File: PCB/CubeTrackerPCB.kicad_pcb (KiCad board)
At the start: 2 copper layers, 28 x 50.9 mm, 9 parts, among them U1 XIAO-RP2040-DIP, U2 ICM-42688-P, U3 DM-OLED096-636

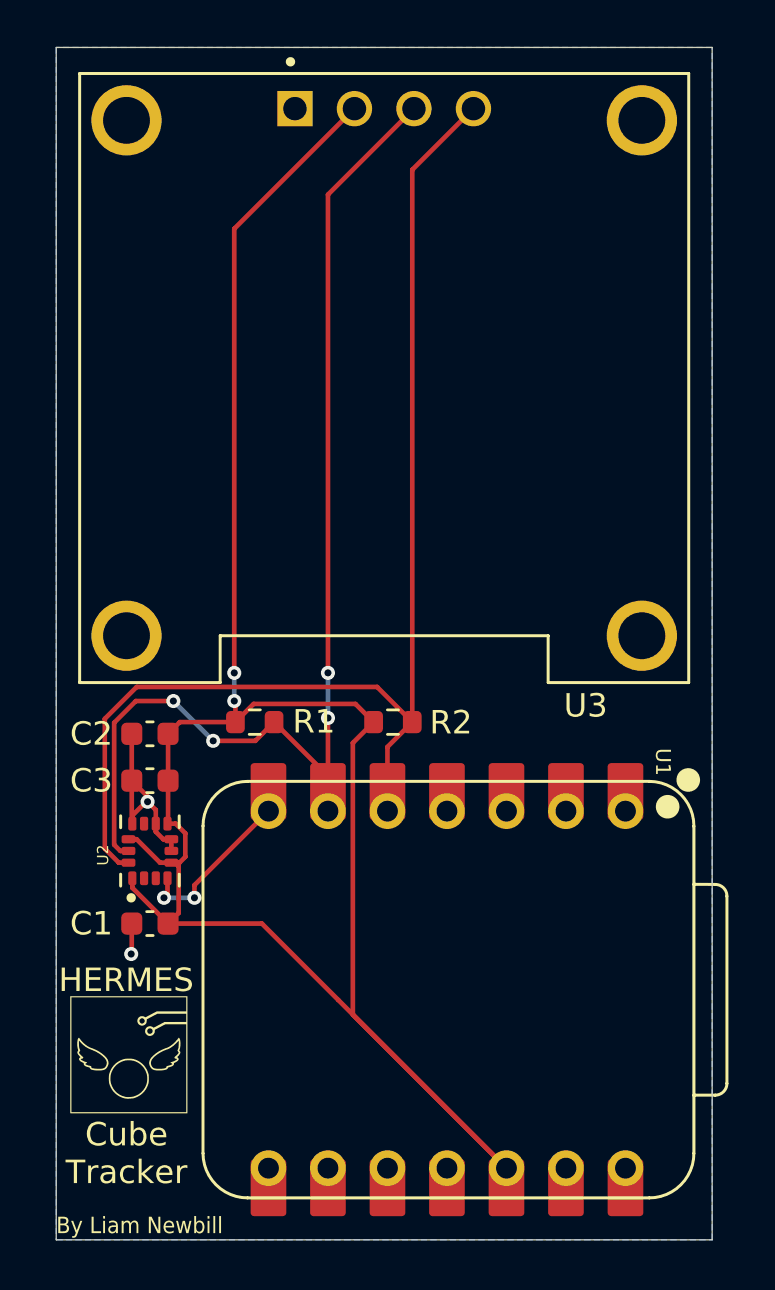
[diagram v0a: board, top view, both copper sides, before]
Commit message: Changed Layout
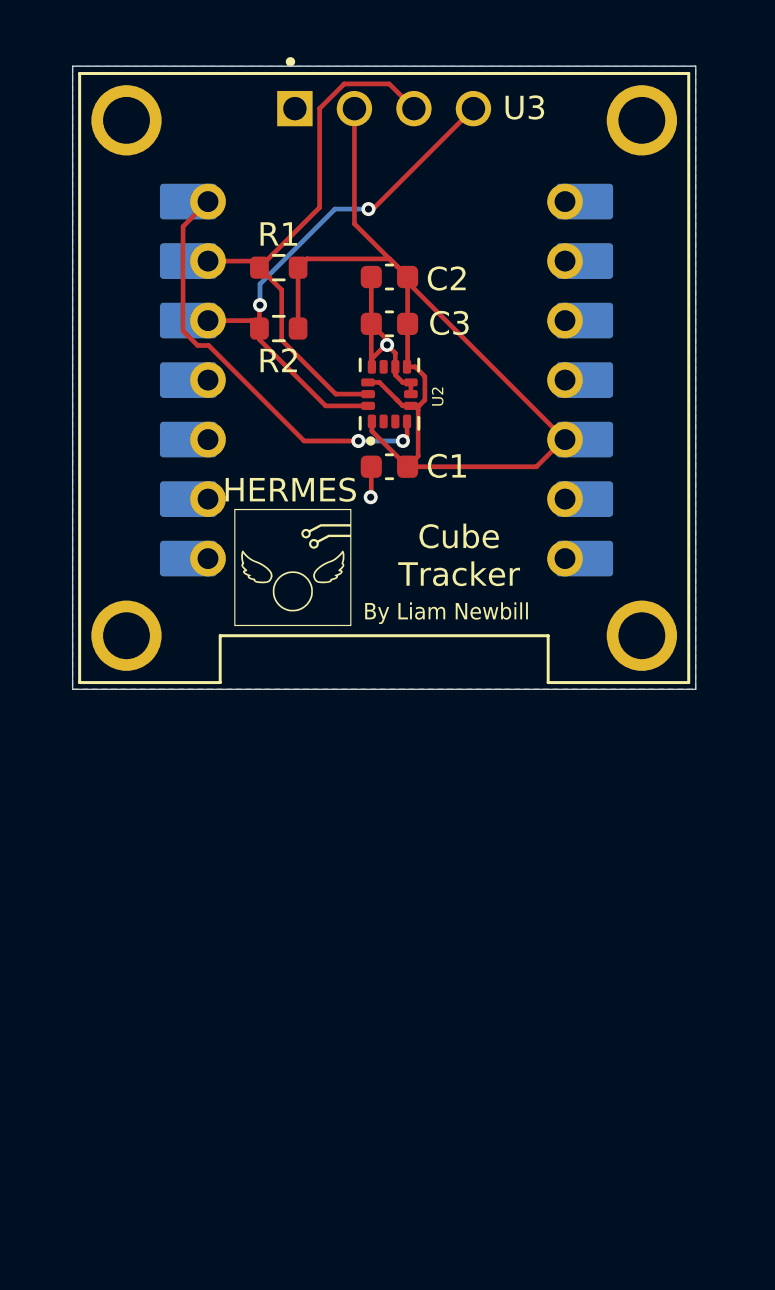
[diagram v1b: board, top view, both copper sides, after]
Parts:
- U1: moved to B.Cu
- moved U1 26.1 mm to (162.1, 63.1), turned to 0 degrees
- moved C1 22.0 mm to (162.2, 66.8)
- moved C2 22.0 mm to (162.2, 58.7)
- moved C3 22.0 mm to (162.2, 60.7)
- moved U2 22.0 mm to (162.2, 63.7)
- moved G*** 21.9 mm to (158.1, 71.1)
- moved R1 19.4 mm to (157.5, 58.3), turned to 0 degrees
- moved R2 17.5 mm to (157.5, 60.9), turned to 180 degrees
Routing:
- net 3.3V: track 93.0 -> 46.9 mm, vias 2 -> 0
- net SDA: track 52.6 -> 22.7 mm, vias 0 -> 2
- net SCL: track 50.4 -> 23.2 mm, vias 4 -> 0
- net ICMINT: track 7.21 -> 18.2 mm
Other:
- board size 28 x 50.9 mm -> 26.6 x 26.6 mm
